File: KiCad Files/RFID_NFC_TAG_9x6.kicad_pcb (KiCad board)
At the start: 2 copper layers, 8.8 x 6.4 mm, 6 parts, among them U1 SL2S2602FTBX

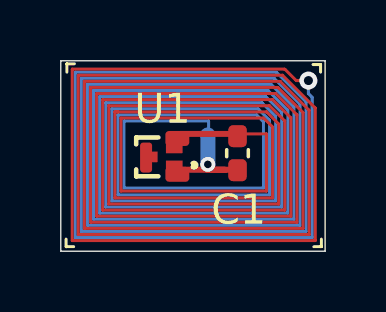
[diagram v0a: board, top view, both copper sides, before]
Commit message: Tag Updates After Testing
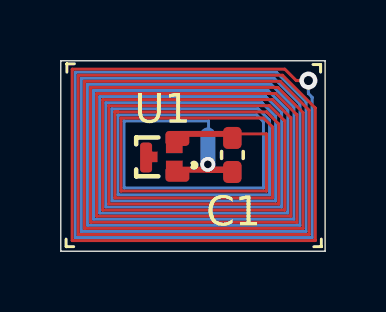
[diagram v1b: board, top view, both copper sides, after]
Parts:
- moved C1 0.18 mm to (133.0, 73.6)
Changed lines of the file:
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@@
 	(footprint "Capacitor_SMD:C_0402_1005Metric_Pad0.74x0.62mm_HandSolder"
 		(layer "F.Cu")
-		(at 133.1722 73.5417 -90)
+		(at 133 73.6 -90)
 		(descr "Capacitor SMD 0402 (1005 Metric), square (rectangular) end terminal, IPC-7351 nominal with elongated pad for handsoldering. (Body size source: IPC-SM-782 page 76, https://www.pcb-3d.com/wordpress/wp-content/uploads/ipc-sm-782a_amendment_1_and_2.pdf), generated with kicad-footprint-generator")
 		(tags "capacitor handsolder")
